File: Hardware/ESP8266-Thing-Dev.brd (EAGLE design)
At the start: 55.4 x 33.8 mm, 84 parts, among them J1 DNP, Q1 MMBT2222A, Q2 MMBT2222A, Q4 BSS138, Q5 BSS138, Q6 BSS138, Q7 BSS138, Q8 BSS138, U1 AP2112K-3.3V, U2 ESP8266, U3 AT25SF041-SOIC8, U4 FTS31XS-U, Y1 26MHz

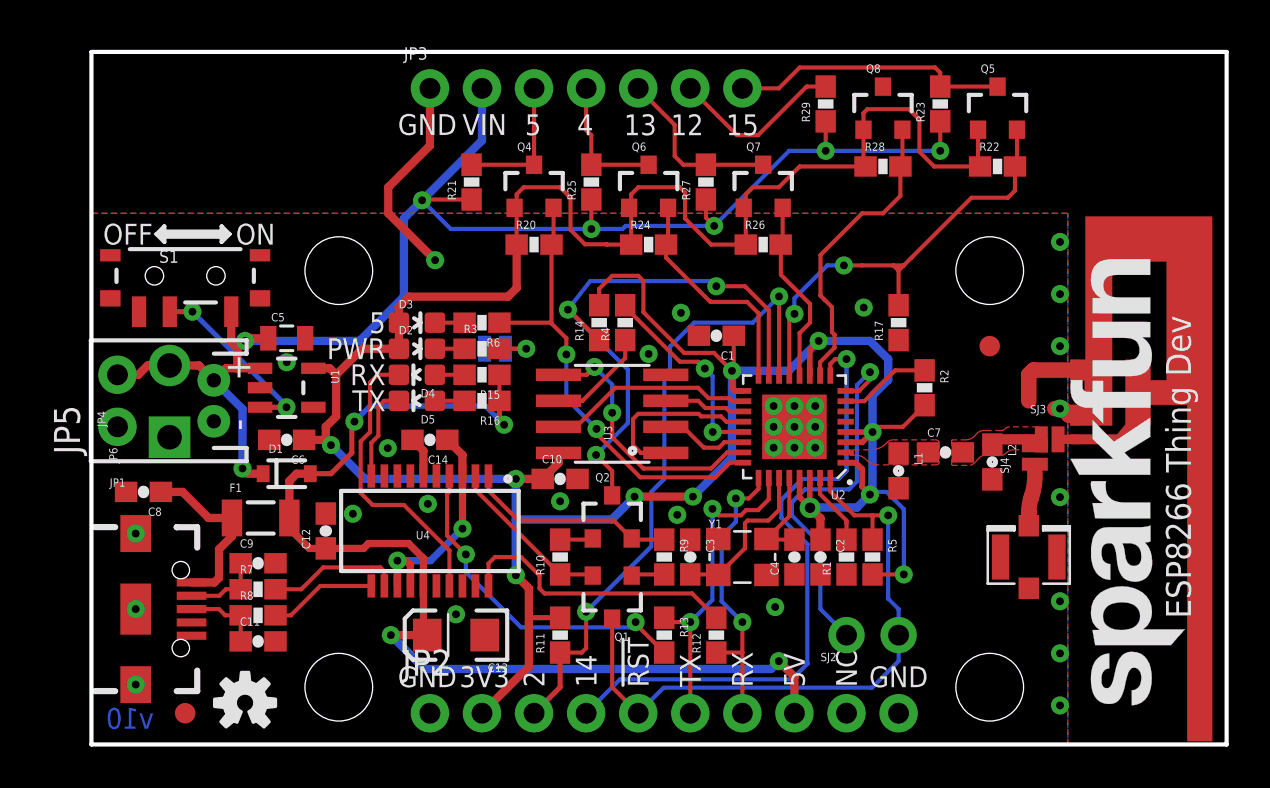
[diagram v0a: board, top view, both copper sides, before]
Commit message: Update gerbs.
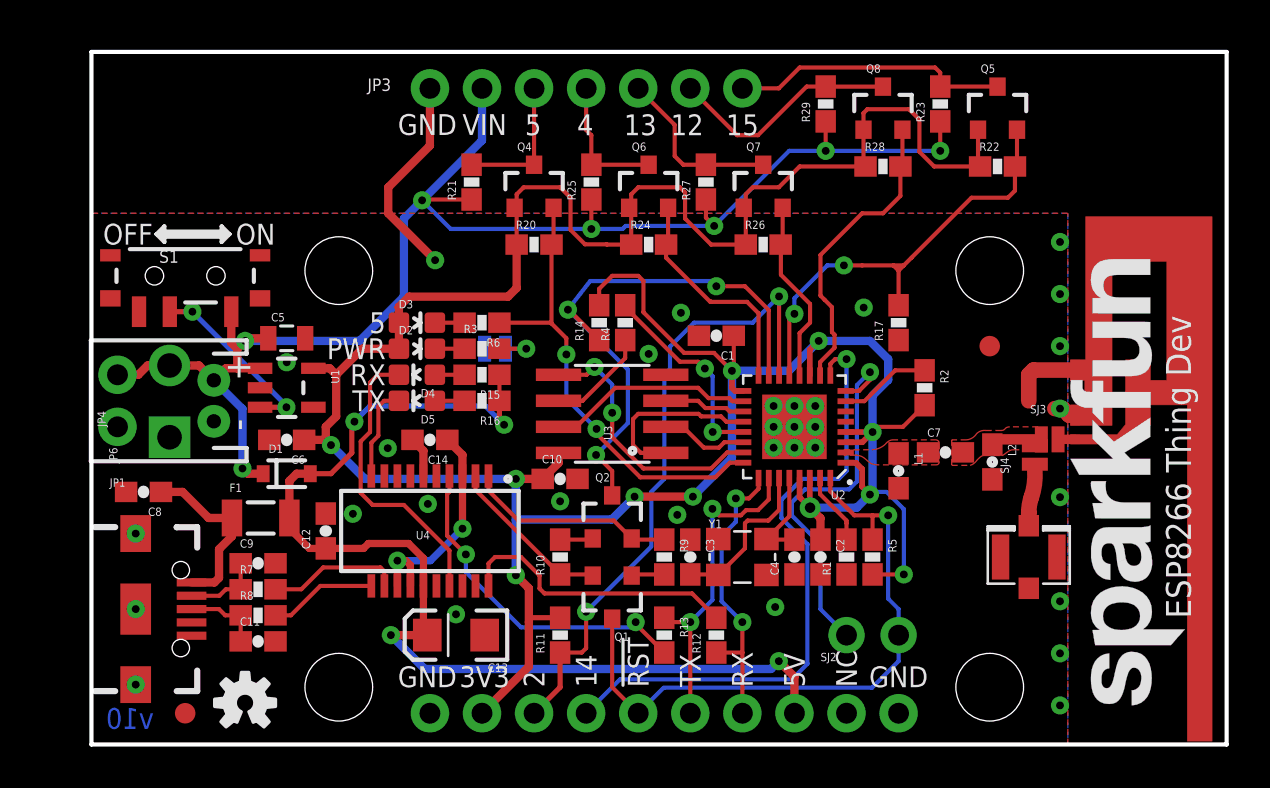
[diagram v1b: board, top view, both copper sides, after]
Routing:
- net GPIO12_OUT: track 8.53 -> 11.3 mm
